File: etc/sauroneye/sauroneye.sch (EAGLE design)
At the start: 9 parts, among them X1 USBSMD

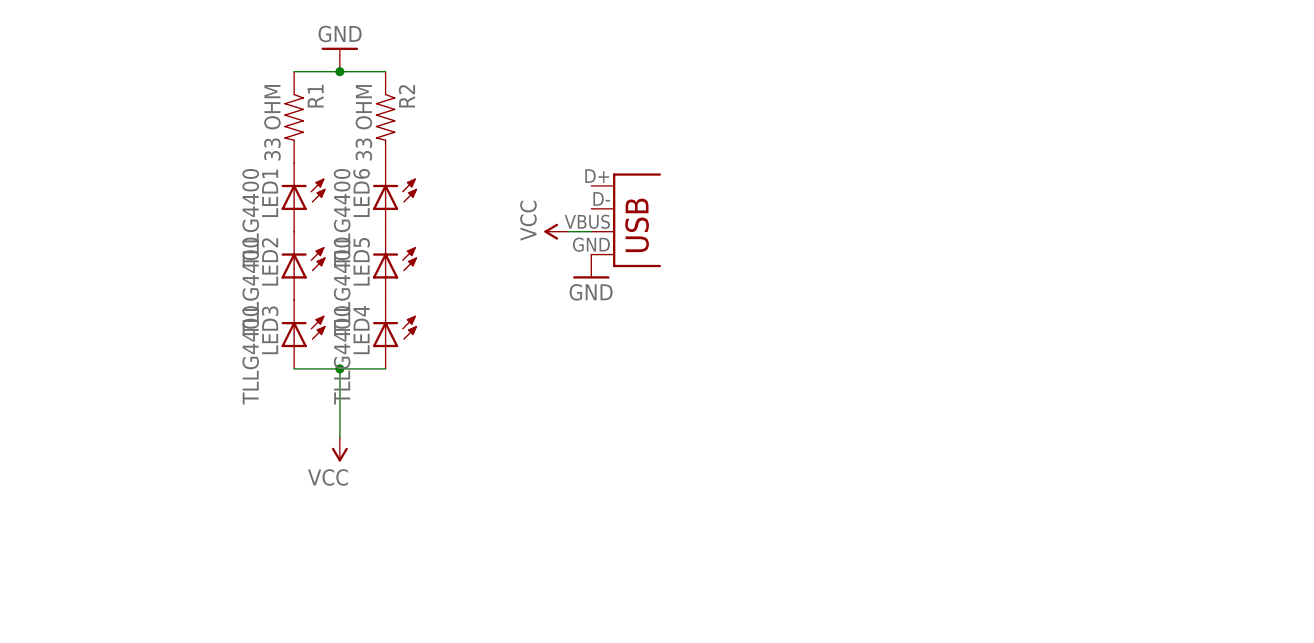
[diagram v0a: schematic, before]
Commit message: new design files from Mark Oehlberg
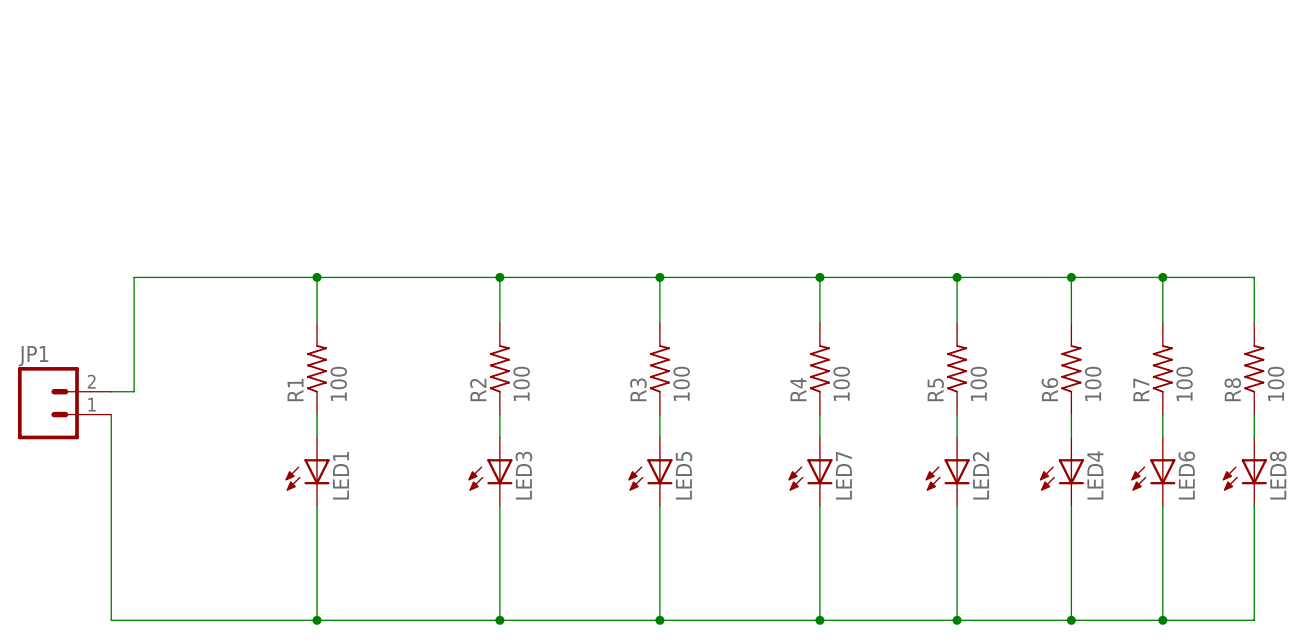
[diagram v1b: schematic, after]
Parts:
- removed X1: USBSMD, SparkFun:USBSMD
- added JP1: (no value), SparkFun-Connectors:M02PTH
- added LED7, LED8: (no value), adafruit:LEDCHIP-LED0805
- added R3, R4, R5, R6, R7, R8: 100, adafruit:R-US_R0805
- LED1, LED2, LED3, LED4, LED5, LED6: value TLLG4400 -> (none); device led:TLLG4400 -> adafruit:LEDCHIP-LED0805
- R1, R2: value 33 OHM -> 100; device SparkFun:RESISTORAXIAL-0.3 -> adafruit:R-US_R0805
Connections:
- removed net GND: R1.1, R2.1, X1.GND
- removed net VCC: LED3.A, LED4.A, X1.VBUS
- new net N$10: LED8.A, R8.1
- new net N$7: LED2.A, R5.1
- new net N$8: LED4.A, R6.1
- new net N$9: LED6.A, R7.1
- net N$1: now also JP1.2, R1.2, R3.2, R4.2, R5.2, R6.2, R7.2, R8.2; no longer LED6.C
- net N$2: now also LED1.A, R1.1; no longer LED1.C, R1.2
- net N$3: now also LED3.A, R2.1; no longer LED5.C, LED6.A
- net N$4: now also R3.1; no longer LED4.C
- net N$5: now also LED7.A, R4.1; no longer LED1.A, LED2.C
- net N$6: now also JP1.1, LED1.C, LED2.C, LED4.C, LED5.C, LED6.C, LED7.C, LED8.C; no longer LED2.A
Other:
- moved on the sheet: LED1, LED2, LED3, LED4, LED5, LED6, R1, R2
